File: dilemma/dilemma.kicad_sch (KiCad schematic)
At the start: 64 parts, among them J1 S3B-PH-SM4-TB(LF)(SN), J2 Serial, J3 BATTERY_CONN_DEANS, J5 S3B-PH-SM4-TB(LF)(SN), J7 trackball, SW1 SW_Push, SW10 SW_Push, SW11 SW_Push, SW12 SW_Push, SW13 SW_Push, SW14 SW_Push, SW15 SW_Push, SW16 SW_Push, SW17 SW_Push, SW2 SW_Push, SW26 SW_SPST, SW3 SW_Push, SW37 SW_SPST, SW4 SW_Push, SW5 SW_Push, SW6 SW_Push, SW7 SW_Push, SW8 SW_Push, SW9 SW_Push, U2 eliteC

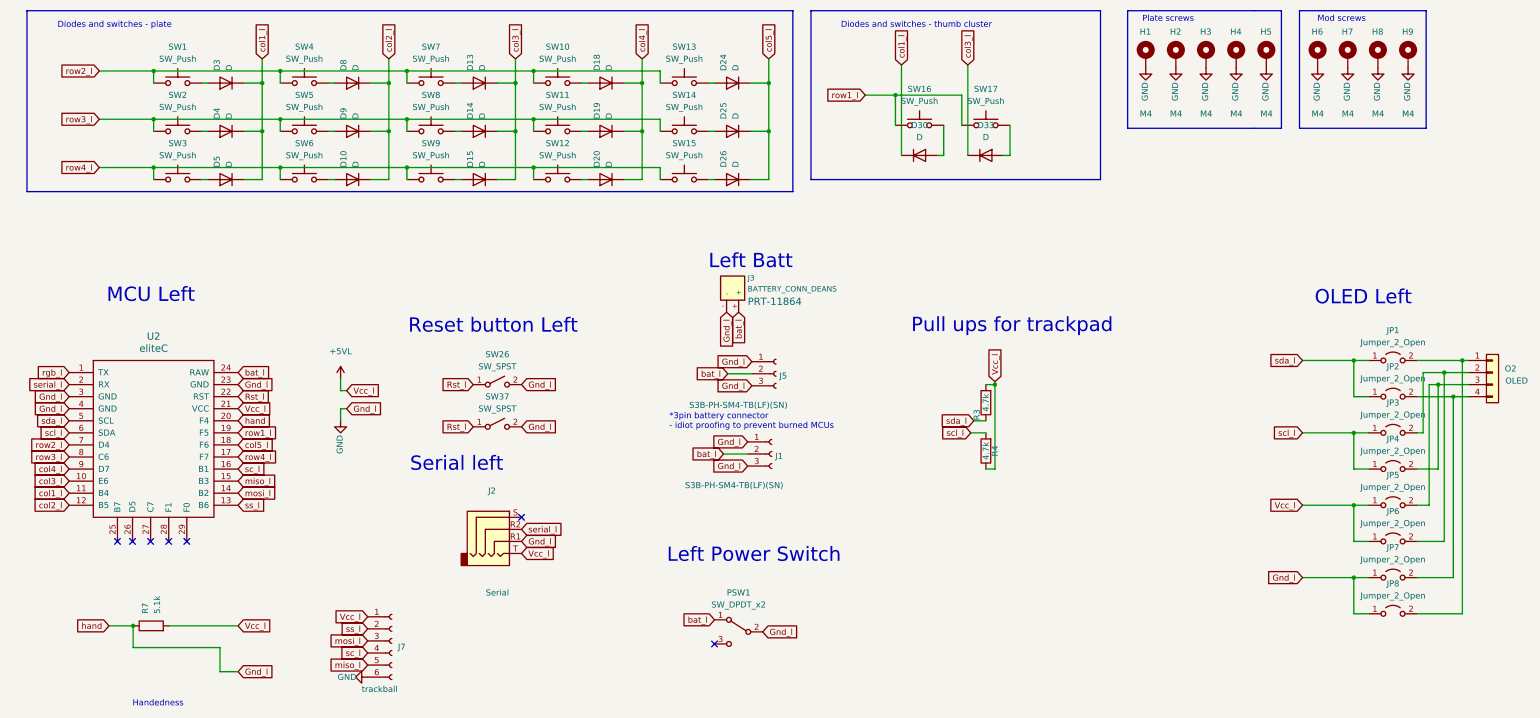
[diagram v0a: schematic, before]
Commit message: routing routing routing
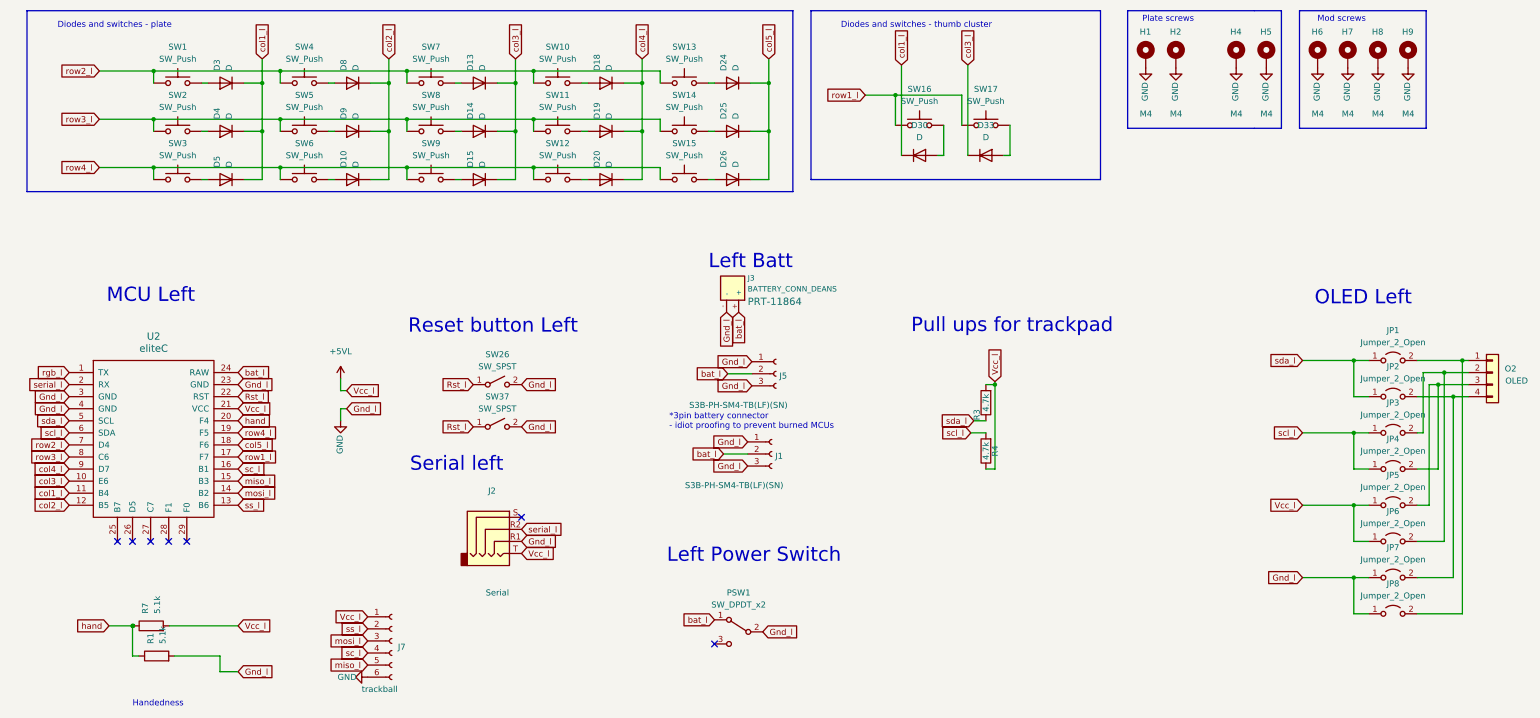
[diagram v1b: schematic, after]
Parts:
- removed H3: M4, footprints:MountingHole_3mm_Pad_thin, symbol Mechanical:MountingHole_Pad
- added R1: 5.1k, footprints:R_1206_handsolder, symbol Device:R
- R7: footprint footprints:R_1206_handsolder_reversible -> footprints:R_1206_handsolder
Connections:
- net GND: now also R1.2; no longer R7.1, U2.20 (F4)
- net row1_l: now also U2.17 (F7); no longer U2.19 (F5)
- net row4_l: now also U2.19 (F5); no longer U2.17 (F7)
- new net hand: R1.1, R7.1, U2.20 (F4)
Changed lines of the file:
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@@
   (junction (at 78.74 48.26) (diameter 0) (color 0 0 0 0)
+  )
+  (junction (at 51.435 152.4) (diameter 0) (color 0 0 0 0)
   )
   (no_connect (at 173.99 156.21))
@@
     (stroke (width 0) (type default) (color 0 0 0 0))
   )
-  (wire (pts (xy 69.85 156.972) (xy 69.85 162.052))
-    (stroke (width 0) (type default) (color 0 0 0 0))
-  )
   (wire (pts (xy 308.61 134.62) (xy 308.61 127))
     (stroke (width 0) (type default) (color 0 0 0 0))
@@
     (stroke (width 0) (type default) (color 0 0 0 0))
   )
-  (wire (pts (xy 46.482 152.4) (xy 51.562 152.4))
+  (wire (pts (xy 46.482 152.4) (xy 51.435 152.4))
     (stroke (width 0) (type default) (color 0 0 0 0))
   )
@@
     (stroke (width 0) (type default) (color 0 0 0 0))
   )
-  (wire (pts (xy 51.562 152.4) (xy 51.562 156.972))
+  (wire (pts (xy 51.435 152.4) (xy 51.435 158.75))
     (stroke (width 0) (type default) (color 0 0 0 0))
   )
@@
     (stroke (width 0) (type default) (color 0 0 0 0))
   )
+  (wire (pts (xy 60.325 158.75) (xy 69.85 158.75))
+    (stroke (width 0) (type default) (color 0 0 0 0))
+  )
   (wire (pts (xy 321.945 119.38) (xy 326.39 119.38))
+    (stroke (width 0) (type default) (color 0 0 0 0))
+  )
+  (wire (pts (xy 51.435 152.4) (xy 51.562 152.4))
     (stroke (width 0) (type default) (color 0 0 0 0))
   )
@@
     (stroke (width 0) (type default) (color 0 0 0 0))
   )
-  (wire (pts (xy 51.562 156.972) (xy 69.85 156.972))
-    (stroke (width 0) (type default) (color 0 0 0 0))
-  )
   (wire (pts (xy 327.66 134.62) (xy 327.66 99.06))
     (stroke (width 0) (type default) (color 0 0 0 0))
   )
   (wire (pts (xy 55.88 48.26) (xy 55.88 45.72))
+    (stroke (width 0) (type default) (color 0 0 0 0))
+  )
+  (wire (pts (xy 69.85 158.75) (xy 69.85 162.052))
     (stroke (width 0) (type default) (color 0 0 0 0))
   )
@@
   )
   (polyline (pts (xy 287.655 22.86) (xy 293.37 22.86))
+    (stroke (width 0) (type default) (color 0 0 0 0))
+  )
+  (wire (pts (xy 52.705 158.75) (xy 51.435 158.75))
     (stroke (width 0) (type default) (color 0 0 0 0))
   )
@@
     )
   )
-  (global_label "row1_l" (shape input) (at 73.66 111.76 0)
-    (effects (font (size 1.27 1.27)) (justify left))
-    (property "Intersheet References" "${INTERSHEET_REFS}" (id 0) (at 102.87 153.67 0)
+  (global_label "row1_l" (shape input) (at 73.66 116.84 0)
+    (effects (font (size 1.27 1.27)) (justify left))
+    (property "Intersheet References" "${INTERSHEET_REFS}" (id 0) (at 102.87 158.75 0)
       (effects (font (size 1.27 1.27)) hide)
     )
@@
     )
   )
-  (global_label "row4_l" (shape input) (at 73.66 116.84 0)
-    (effects (font (size 1.27 1.27)) (justify left))
-    (property "Intersheet References" "${INTERSHEET_REFS}" (id 0) (at 102.87 171.45 0)
+  (global_label "row4_l" (shape input) (at 73.66 111.76 0)
+    (effects (font (size 1.27 1.27)) (justify left))
+    (property "Intersheet References" "${INTERSHEET_REFS}" (id 0) (at 102.87 166.37 0)
       (effects (font (size 1.27 1.27)) hide)
     )
@@
       (effects (font (size 1.27 1.27)) (justify left))
     )
-    (property "Footprint" "footprints:R_1206_handsolder_reversible" (id 2) (at 55.372 154.178 90)
+    (property "Footprint" "footprints:R_1206_handsolder" (id 2) (at 55.372 154.178 90)
       (effects (font (size 1.27 1.27)) hide)
     )
@@
     (pin "2")
   )
+  (symbol (lib_id "Device:R") (at 56.515 158.75 90) (unit 1)
+    (in_bom yes) (on_board yes)
+    (property "Reference" "R1" (id 0) (at 55.245 156.21 0)
+      (effects (font (size 1.27 1.27)) (justify left))
+    )
+    (property "Value" "5.1k" (id 1) (at 57.785 156.21 0)
+      (effects (font (size 1.27 1.27)) (justify left))
+    )
+    (property "Footprint" "footprints:R_1206_handsolder" (id 2) (at 56.515 160.528 90)
+      (effects (font (size 1.27 1.27)) hide)
+    )
+    (property "Datasheet" "~" (id 3) (at 56.515 158.75 0)
+      (effects (font (size 1.27 1.27)) hide)
+    )
+    (property "JLCPCB BOM" "1" (id 4) (at 56.515 158.75 0)
+      (effects (font (size 1.27 1.27)) hide)
+    )
+    (property "JLCPCB Part" "C26033" (id 5) (at 56.515 158.75 0)
+      (effects (font (size 1.27 1.27)) hide)
+    )
+    (pin "1")
+    (pin "2")
+  )
   (symbol (lib_id "Device:D") (at 151.13 38.1 180) (unit 1)
     (in_bom yes) (on_board yes)
@@
     (pin "2")
   )
-  (symbol (lib_id "power:GND") (at 277.495 34.925 0) (unit 1)
-    (in_bom yes) (on_board yes)
-    (property "Reference" "#PWR0107" (id 0) (at 277.495 41.275 0)
-      (effects (font (size 1.27 1.27)) hide)
-    )
-    (property "Value" "GND" (id 1) (at 277.339 41.9099 90)
-      (effects (font (size 1.27 1.27)) (justify left))
-    )
-    (property "Footprint" "" (id 2) (at 277.495 34.925 0)
-      (effects (font (size 1.27 1.27)) hide)
-    )
-    (property "Datasheet" "" (id 3) (at 277.495 34.925 0)
-      (effects (font (size 1.27 1.27)) hide)
-    )
-    (pin "1")
-  )
   (symbol (lib_id "power:+5VL") (at 95.25 100.33 0) (unit 1)
     (in_bom yes) (on_board yes) (fields_autoplaced)
@@
     )
     (property "Datasheet" "" (id 3) (at 307.34 34.925 0)
-      (effects (font (size 1.27 1.27)) hide)
-    )
-    (pin "1")
-  )
-  (symbol (lib_id "Mechanical:MountingHole_Pad") (at 277.495 32.385 0) (unit 1)
-    (in_bom yes) (on_board yes)
-    (property "Reference" "H3" (id 0) (at 276.225 27.305 0)
-      (effects (font (size 1.27 1.27)) (justify left))
-    )
-    (property "Value" "M4" (id 1) (at 276.225 44.577 0)
-      (effects (font (size 1.27 1.27)) (justify left))
-    )
-    (property "Footprint" "footprints:MountingHole_3mm_Pad_thin" (id 2) (at 277.495 32.385 0)
-      (effects (font (size 1.27 1.27)) hide)
-    )
-    (property "Datasheet" "~" (id 3) (at 277.495 32.385 0)
       (effects (font (size 1.27 1.27)) hide)
     )
@@
       (reference "#PWR0106") (unit 1) (value "GND") (footprint "")
     )
-    (path "/7ee12246-48f8-49a8-bcd4-e3487c6db589"
-      (reference "#PWR0107") (unit 1) (value "GND") (footprint "")
-    )
     (path "/bacc65b4-66ed-4f84-a32f-72178fa6b135"
       (reference "D3") (unit 1) (value "D") (footprint "footprints:D_1206_handsolder_reversible")
@@
       (reference "H2") (unit 1) (value "M4") (footprint "footprints:MountingHole_3mm_Pad_thin")
     )
-    (path "/8f3d2726-b39f-482d-888f-43d8200309de"
-      (reference "H3") (unit 1) (value "M4") (footprint "footprints:MountingHole_3mm_Pad_thin")
-    )
     (path "/eab541c6-214e-4bdc-a65e-96cf56f5a486"
       (reference "H4") (unit 1) (value "M4") (footprint "footprints:MountingHole_3mm_Pad_thin")
@@
       (reference "PSW1") (unit 1) (value "SW_DPDT_x2") (footprint "local-libraries:Switch_MSK-12C01-07")
     )
+    (path "/4472aae1-b147-4122-a247-84cbdd93496c"
+      (reference "R1") (unit 1) (value "5.1k") (footprint "footprints:R_1206_handsolder")
+    )
     (path "/4acaff23-3513-4df1-ad8e-582535069bb0"
       (reference "R3") (unit 1) (value "4.7k") (footprint "footprints:R_1206_handsolder_reversible")
@@
     )
     (path "/230e74d0-be4c-4179-b8ac-0a56b1c74f86"
-      (reference "R7") (unit 1) (value "5.1k") (footprint "footprints:R_1206_handsolder_reversible")
+      (reference "R7") (unit 1) (value "5.1k") (footprint "footprints:R_1206_handsolder")
     )
     (path "/10c00776-633d-4d70-8200-26e4b25fd090"
